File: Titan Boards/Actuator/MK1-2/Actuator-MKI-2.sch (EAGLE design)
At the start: 68 parts, among them Q10 MOSFET-NCH-AO3404A, Q12 MOSFET-NCH-AO3404A, Q13 MOSFET-NCH-AO3404A, Q14 MOSFET-NCH-AO3404A, Q17 MOSFET-NCH-AO3404A, Q18 FDD4141TO252, Q19 MOSFET-NCH-AO3404A, Q2 MOSFET-NCH-AO3404A, Q20 MOSFET-NCH-AO3404A, Q3 MOSFET-NCH-AO3404A, Q4 MOSFET-NCH-AO3404A, Q5 MOSFET-NCH-AO3404A, Q6 FDD4141TO252, Q7 MOSFET-NCH-AO3404A, Q8 MOSFET-NCH-AO3404A, Q9 MOSFET-NCH-AO3404A, U1 DRV8816PWPR

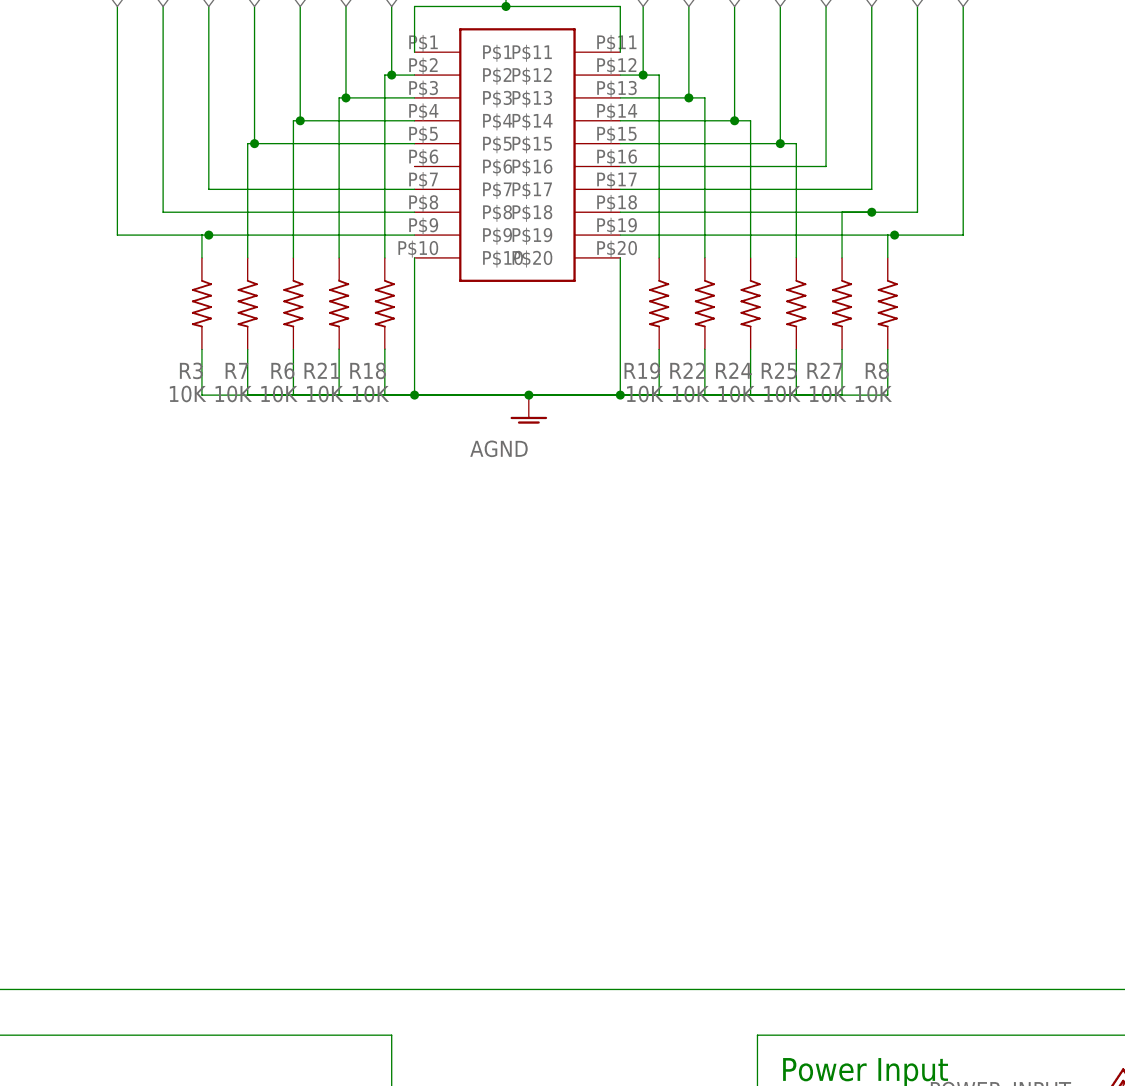
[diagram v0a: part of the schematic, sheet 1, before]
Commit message: Actuator Mk1-2 Updates
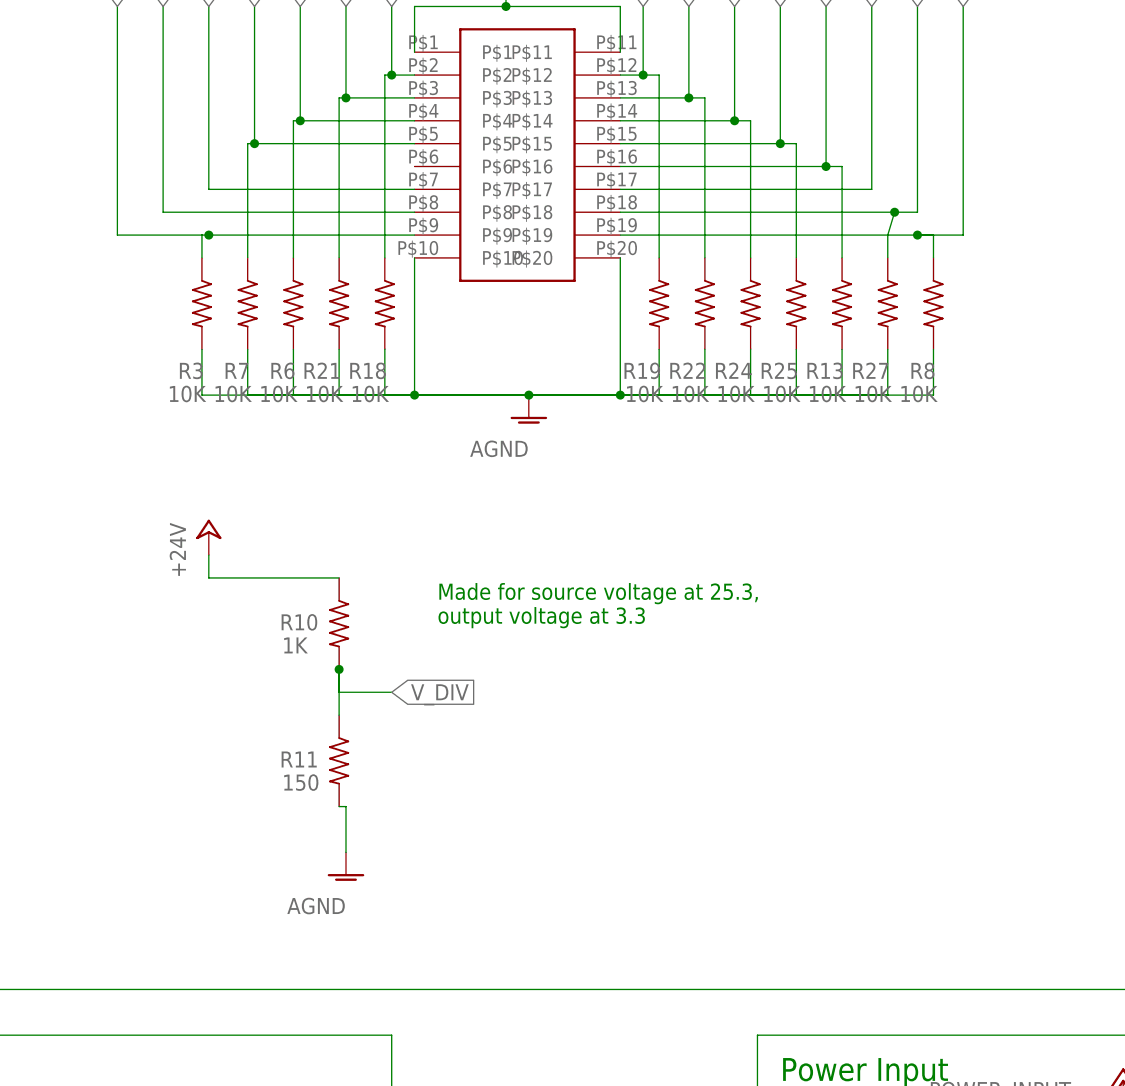
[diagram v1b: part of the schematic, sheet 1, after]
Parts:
- added R10: 1K, resistor:R-US_R0603
- added R11: 150, resistor:R-US_R0603
- added R13: 10K, resistor:R-US_R0603
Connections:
- net +24V: now also R10.1
- net AGND: now also R11.2, R13.2
- net MOTOR_EN: now also R13.1
- net V_DIV: now also R10.2, R11.1
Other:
- note added: "Made for source voltage at 25.3, output voltage at 3.3"
- moved on the sheet: R27, R8
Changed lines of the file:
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@@
 <part name="R8" library="resistor" library_urn="urn:adsk.eagle:library:348" deviceset="R-US_" device="R0603" package3d_urn="urn:adsk.eagle:package:23555/2" value="10K"/>
 <part name="P+2" library="supply1" library_urn="urn:adsk.eagle:library:371" deviceset="V+" device=""/>
+<part name="P+11" library="supply1" library_urn="urn:adsk.eagle:library:371" deviceset="+24V" device=""/>
+<part name="R10" library="resistor" library_urn="urn:adsk.eagle:library:348" deviceset="R-US_" device="R0603" package3d_urn="urn:adsk.eagle:package:23555/2" value="1K"/>
+<part name="R11" library="resistor" library_urn="urn:adsk.eagle:library:348" deviceset="R-US_" device="R0603" package3d_urn="urn:adsk.eagle:package:23555/2" value="150"/>
+<part name="AGND1" library="supply1" library_urn="urn:adsk.eagle:library:371" deviceset="AGND" device=""/>
+<part name="R13" library="resistor" library_urn="urn:adsk.eagle:library:348" deviceset="R-US_" device="R0603" package3d_urn="urn:adsk.eagle:package:23555/2" value="10K"/>
 </parts>
 <sheets>
@@
 electrolytic
 bulk capacitor.</text>
+<text x="289.56" y="96.52" size="1.778" layer="91">Made for source voltage at 25.3,
+output voltage at 3.3</text>
 </plain>
 <instances>
@@
 <attribute name="VALUE" x="325.628" y="121.158" size="1.778" layer="96"/>
 </instance>
-<instance part="R27" gate="G$1" x="334.518" y="132.08" smashed="yes" rot="R270">
-<attribute name="NAME" x="334.772" y="125.5014" size="1.778" layer="95" rot="R180"/>
-<attribute name="VALUE" x="330.708" y="121.158" size="1.778" layer="96"/>
+<instance part="R27" gate="G$1" x="339.598" y="132.08" smashed="yes" rot="R270">
+<attribute name="NAME" x="339.852" y="125.5014" size="1.778" layer="95" rot="R180"/>
+<attribute name="VALUE" x="335.788" y="121.158" size="1.778" layer="96"/>
 </instance>
 <instance part="R3" gate="G$1" x="263.398" y="132.08" smashed="yes" rot="R270">
@@
 <attribute name="VALUE" x="259.588" y="121.158" size="1.778" layer="96"/>
 </instance>
-<instance part="R8" gate="G$1" x="339.598" y="132.08" smashed="yes" rot="R270">
-<attribute name="NAME" x="339.852" y="125.5014" size="1.778" layer="95" rot="R180"/>
-<attribute name="VALUE" x="335.788" y="121.158" size="1.778" layer="96"/>
+<instance part="R8" gate="G$1" x="344.678" y="132.08" smashed="yes" rot="R270">
+<attribute name="NAME" x="344.932" y="125.5014" size="1.778" layer="95" rot="R180"/>
+<attribute name="VALUE" x="340.868" y="121.158" size="1.778" layer="96"/>
 </instance>
 <instance part="P+2" gate="1" x="274.32" y="43.18" smashed="yes">
 <attribute name="VALUE" x="271.78" y="40.64" size="1.778" layer="96" rot="R90"/>
 </instance>
+<instance part="P+11" gate="1" x="264.16" y="106.68" smashed="yes">
+<attribute name="VALUE" x="261.62" y="101.6" size="1.778" layer="96" rot="R90"/>
+</instance>
+<instance part="R10" gate="G$1" x="278.638" y="96.52" smashed="yes" rot="R270">
+<attribute name="NAME" x="276.352" y="97.5614" size="1.778" layer="95" rot="R180"/>
+<attribute name="VALUE" x="272.288" y="93.218" size="1.778" layer="96"/>
+</instance>
+<instance part="R11" gate="G$1" x="278.638" y="81.28" smashed="yes" rot="R270">
+<attribute name="NAME" x="276.352" y="82.3214" size="1.778" layer="95" rot="R180"/>
+<attribute name="VALUE" x="272.288" y="77.978" size="1.778" layer="96"/>
+</instance>
+<instance part="AGND1" gate="VR1" x="279.4" y="68.58" smashed="yes">
+<attribute name="VALUE" x="279.4" y="66.04" size="1.778" layer="96" rot="R180"/>
+</instance>
+<instance part="R13" gate="G$1" x="334.518" y="132.08" smashed="yes" rot="R270">
+<attribute name="NAME" x="334.772" y="125.5014" size="1.778" layer="95" rot="R180"/>
+<attribute name="VALUE" x="330.708" y="121.158" size="1.778" layer="96"/>
+</instance>
 </instances>
 <busses>
@@
 <wire x1="329.438" y1="121.92" x2="309.88" y2="121.92" width="0.1524" layer="91"/>
 <pinref part="R27" gate="G$1" pin="2"/>
-<wire x1="334.518" y1="127" x2="334.518" y2="121.92" width="0.1524" layer="91"/>
-<wire x1="334.518" y1="121.92" x2="309.88" y2="121.92" width="0.1524" layer="91"/>
+<wire x1="339.598" y1="127" x2="339.598" y2="121.92" width="0.1524" layer="91"/>
+<wire x1="339.598" y1="121.92" x2="309.88" y2="121.92" width="0.1524" layer="91"/>
 <pinref part="R3" gate="G$1" pin="2"/>
 <wire x1="263.398" y1="127" x2="263.398" y2="121.92" width="0.1524" layer="91"/>
 <wire x1="263.398" y1="121.92" x2="299.72" y2="121.92" width="0.1524" layer="91"/>
 <pinref part="R8" gate="G$1" pin="2"/>
-<wire x1="339.598" y1="127" x2="339.598" y2="121.92" width="0.1524" layer="91"/>
-<wire x1="339.598" y1="121.92" x2="299.72" y2="121.92" width="0.1524" layer="91"/>
+<wire x1="344.678" y1="127" x2="344.678" y2="121.92" width="0.1524" layer="91"/>
+<wire x1="344.678" y1="121.92" x2="299.72" y2="121.92" width="0.1524" layer="91"/>
+<pinref part="R13" gate="G$1" pin="2"/>
+<wire x1="334.518" y1="127" x2="334.518" y2="121.92" width="0.1524" layer="91"/>
+<wire x1="334.518" y1="121.92" x2="299.72" y2="121.92" width="0.1524" layer="91"/>
 </segment>
 <segment>
@@
 <junction x="172.72" y="17.78"/>
 </segment>
+<segment>
+<pinref part="R11" gate="G$1" pin="2"/>
+<pinref part="AGND1" gate="VR1" pin="AGND"/>
+<wire x1="278.638" y1="76.2" x2="279.4" y2="76.2" width="0.1524" layer="91"/>
+<wire x1="279.4" y1="76.2" x2="279.4" y2="71.12" width="0.1524" layer="91"/>
+</segment>
 </net>
 <net name="SDA" class="0">
@@
 <wire x1="116.84" y1="185.42" x2="116.84" y2="187.96" width="0.1524" layer="91"/>
 </segment>
+<segment>
+<pinref part="R10" gate="G$1" pin="1"/>
+<pinref part="P+11" gate="1" pin="+24V"/>
+<wire x1="278.638" y1="101.6" x2="264.16" y2="101.6" width="0.1524" layer="91"/>
+<wire x1="264.16" y1="101.6" x2="264.16" y2="104.14" width="0.1524" layer="91"/>
+</segment>
 </net>
 <net name="N$4" class="0">
@@
 <pinref part="R27" gate="G$1" pin="1"/>
 <pinref part="U$9" gate="G$1" pin="P$18"/>
-<wire x1="334.518" y1="137.16" x2="334.518" y2="142.24" width="0.1524" layer="91"/>
-<wire x1="334.518" y1="142.24" x2="337.82" y2="142.24" width="0.1524" layer="91"/>
-<wire x1="337.82" y1="142.24" x2="309.88" y2="142.24" width="0.1524" layer="91"/>
-<wire x1="337.82" y1="142.24" x2="342.9" y2="142.24" width="0.1524" layer="91"/>
+<wire x1="339.598" y1="137.16" x2="339.598" y2="139.7" width="0.1524" layer="91"/>
+<wire x1="339.598" y1="139.7" x2="340.36" y2="142.24" width="0.1524" layer="91"/>
+<wire x1="340.36" y1="142.24" x2="309.88" y2="142.24" width="0.1524" layer="91"/>
+<wire x1="340.36" y1="142.24" x2="342.9" y2="142.24" width="0.1524" layer="91"/>
 <wire x1="342.9" y1="142.24" x2="342.9" y2="165.1" width="0.1524" layer="91"/>
-<junction x="337.82" y="142.24"/>
+<junction x="340.36" y="142.24"/>
 <label x="342.9" y="165.1" size="1.778" layer="95" rot="R90" xref="yes"/>
 </segment>
@@
 <label x="347.98" y="165.1" size="1.778" layer="95" rot="R90" xref="yes"/>
 <pinref part="U$9" gate="G$1" pin="P$19"/>
-<wire x1="347.98" y1="139.7" x2="340.36" y2="139.7" width="0.1524" layer="91"/>
+<wire x1="347.98" y1="139.7" x2="342.9" y2="139.7" width="0.1524" layer="91"/>
 <pinref part="R8" gate="G$1" pin="1"/>
-<wire x1="339.598" y1="139.7" x2="309.88" y2="139.7" width="0.1524" layer="91"/>
-<wire x1="339.598" y1="137.16" x2="339.598" y2="139.7" width="0.1524" layer="91"/>
-<wire x1="339.598" y1="139.7" x2="340.36" y2="139.7" width="0.1524" layer="91"/>
-<junction x="340.36" y="139.7"/>
+<wire x1="342.9" y1="139.7" x2="309.88" y2="139.7" width="0.1524" layer="91"/>
+<wire x1="344.678" y1="137.16" x2="344.678" y2="139.7" width="0.1524" layer="91"/>
+<wire x1="344.678" y1="139.7" x2="342.9" y2="139.7" width="0.1524" layer="91"/>
+<junction x="342.9" y="139.7"/>
 </segment>
 </net>
@@
 <label x="259.08" y="165.1" size="1.778" layer="95" rot="R90" xref="yes"/>
 </segment>
+<segment>
+<wire x1="278.638" y1="88.9" x2="284.48" y2="88.9" width="0.1524" layer="91"/>
+<label x="284.48" y="88.9" size="1.778" layer="95" xref="yes"/>
+<pinref part="R11" gate="G$1" pin="1"/>
+<pinref part="R10" gate="G$1" pin="2"/>
+<wire x1="278.638" y1="86.36" x2="278.638" y2="91.44" width="0.1524" layer="91"/>
+<wire x1="278.638" y1="88.9" x2="278.638" y2="91.44" width="0.1524" layer="91"/>
+<junction x="278.638" y="91.44"/>
+</segment>
 </net>
 <net name="MOTOR_EN" class="0">
@@
 <wire x1="332.74" y1="147.32" x2="332.74" y2="165.1" width="0.1524" layer="91"/>
 <label x="332.74" y="165.1" size="1.778" layer="95" rot="R90" xref="yes"/>
+<pinref part="R13" gate="G$1" pin="1"/>
+<wire x1="334.518" y1="137.16" x2="334.518" y2="147.32" width="0.1524" layer="91"/>
+<wire x1="334.518" y1="147.32" x2="332.74" y2="147.32" width="0.1524" layer="91"/>
+<junction x="332.74" y="147.32"/>
 </segment>
 <segment>
